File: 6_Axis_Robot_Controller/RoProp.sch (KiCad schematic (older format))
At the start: 31 parts

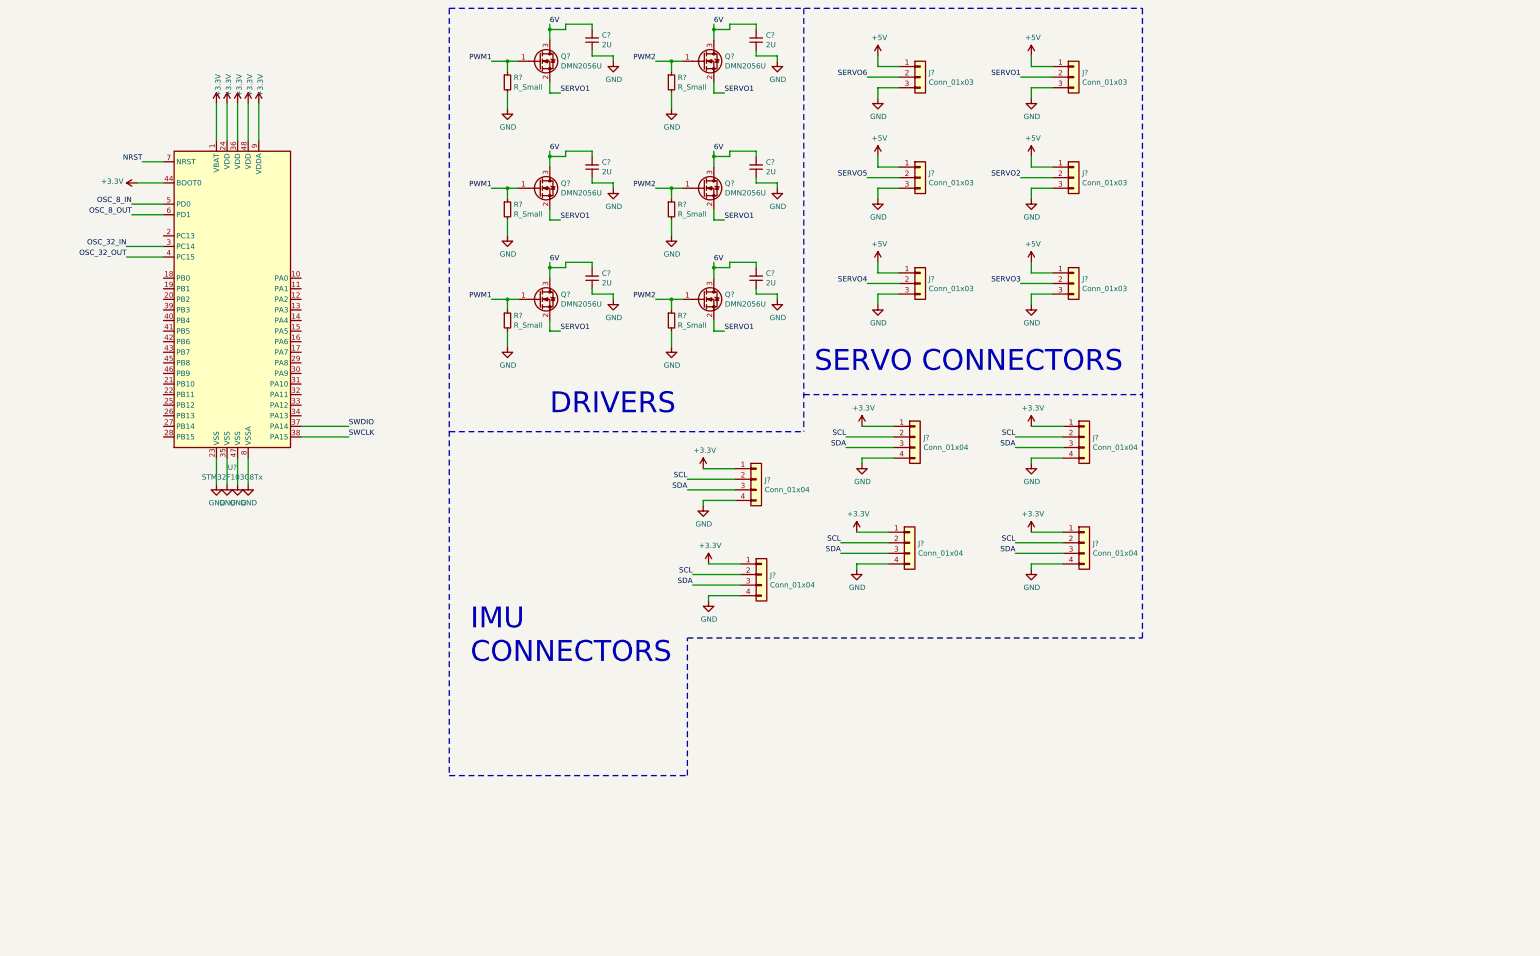
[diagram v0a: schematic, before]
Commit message: Add files via upload
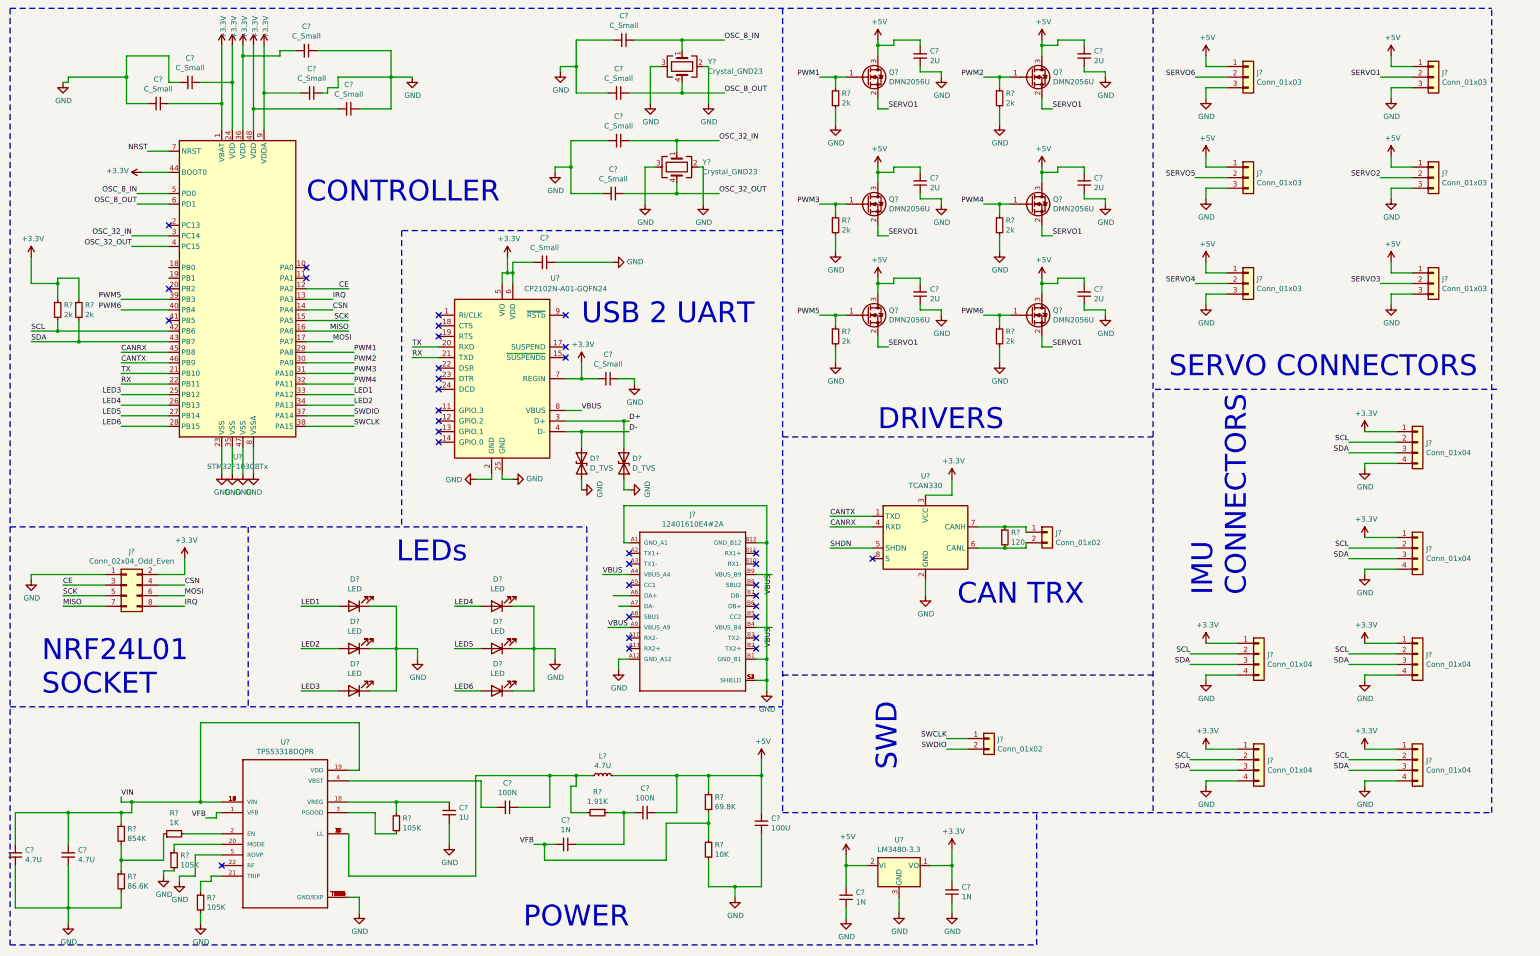
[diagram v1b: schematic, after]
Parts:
- added C? (x5): C_Small, Capacitor_SMD:C_0402_1005Metric, symbol Device:C_Small
- added C? (x2): 100N, symbol Device:C_Small
- added C? (x3): 1N, symbol Device:C_Small
- added C?: 100U, symbol Device:C_Small
- added C? (x2): 4.7U, symbol Device:C_Small
- added C?: 1U, symbol Device:C_Small
- added C? (x6): C_Small, symbol Device:C_Small
- added D? (x2): D_TVS, symbol Device:D_TVS
- added D? (x6): LED, symbol Device:LED
- added J? (x2): Conn_01x02, Connector_JST:JST_PH_B2B-PH-K_1x02_P2.00mm_Vertical, symbol Connector_Generic:Conn_01x02
- added J?: 12401610E4#2A, AMPHENOL_12401610E4#2A, symbol K_USB_C_receptacle:12401610E4#2A
- added J?: Conn_02x04_Odd_Even, symbol Connector_Generic:Conn_02x04_Odd_Even
- added L?: 4.7U, symbol Device:L_Small
- added R? (x2): 2k, Resistor_SMD:R_0805_2012Metric_Pad1.15x1.40mm_HandSolder, symbol Device:R_Small
- added R?: 1.91K, symbol Device:R_Small
- added R?: 69.8K, symbol Device:R_Small
- added R?: 10K, symbol Device:R_Small
- added R?: 1K, symbol Device:R_Small
- added R?: 854K, symbol Device:R_Small
- added R?: 86.6K, symbol Device:R_Small
- added R? (x3): 105K, symbol Device:R_Small
- added R?: 120, symbol Device:R_Small
- added U?: TPS53318DQPR, CONV_TPS53318DQPR, symbol K_TPS53318DQPR:TPS53318DQPR
- added U?: LM3480-3.3, Package_TO_SOT_SMD:SOT-23, symbol Regulator_Linear:LM3480-3.3
- added U?: TCAN330, symbol Interface_CAN_LIN:TCAN330
- added U?: CP2102N-A01-GQFN24, Package_DFN_QFN:QFN-24-1EP_4x4mm_P0.5mm_EP2.6x2.6mm, symbol Interface_USB:CP2102N-A01-GQFN24
- added Y? (x2): Crystal_GND23, symbol Device:Crystal_GND23
- R? (x6): value R_Small -> 2k
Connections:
- net 6V is gone; now on net +5V: C?.2, C?.2, C?.2, C?.2, C?.2, C?.2, Q?.3 (D), Q?.3 (D), Q?.3 (D), Q?.3 (D), Q?.3 (D), Q?.3 (D)
- net +3V3: now also C?.1, C?.1, C?.2, C?.2, C?.2, C?.2, C?.2, C?.2, J?.2 (Pin_2), R?.1, R?.1, U?.1 (VO), U?.3 (VCC), U?.5 (VIO), U?.6 (VDD), U?.7 (REGIN)
- net +5V: now also C?.1, C?.2, C?.2, L?.2, R?.2, U?.2 (VI)
- net GND: now also C?.1, C?.1, C?.1, C?.1, C?.1, C?.1, C?.1, C?.1, C?.1, C?.1, C?.1, C?.2, C?.2, C?.2, C?.2, C?.2, C?.2, D?.1 (K), D?.1 (K), D?.1 (K), D?.1 (K), D?.1 (K), D?.1 (K), D?.2 (A2), D?.2 (A2), J?.1 (Pin_1), J?.A1 (GND_A1), J?.A12 (GND_A12), J?.B1 (GND_B1), J?.B12 (GND_B12), J?.S1 (SHIELD), J?.S2 (SHIELD), J?.S3 (SHIELD), J?.S4 (SHIELD), R?.1, R?.2, R?.2, R?.2, U?.2 (GND), U?.2 (GND), U?.23 (GND/EXP), U?.25 (GND), U?.3 (GND), U?.5 (ROVP), U?.TV1 (GND/EXP), U?.TV10 (GND/EXP), U?.TV11 (GND/EXP), U?.TV12 (GND/EXP), U?.TV13 (GND/EXP), U?.TV14 (GND/EXP), U?.TV15 (GND/EXP), U?.TV16 (GND/EXP), U?.TV17 (GND/EXP), U?.TV18 (GND/EXP), U?.TV19 (GND/EXP), U?.TV2 (GND/EXP), U?.TV20 (GND/EXP), U?.TV21 (GND/EXP), U?.TV3 (GND/EXP), U?.TV4 (GND/EXP), U?.TV5 (GND/EXP), U?.TV6 (GND/EXP), U?.TV7 (GND/EXP), U?.TV8 (GND/EXP), U?.TV9 (GND/EXP), Y?.2, Y?.2, Y?.3, Y?.3
- net OSC_32_IN: now also C?.1, Y?.1
- net OSC_32_OUT: now also C?.1, Y?.4
- net OSC_8_IN: now also C?.1, Y?.1
- net OSC_8_OUT: now also C?.1, Y?.4
- net PWM1: now also U?.29 (PA8); no longer Q?.1 (G), Q?.1 (G), R?.1, R?.1
- net PWM2: now also U?.30 (PA9); no longer Q?.1 (G), Q?.1 (G), R?.1, R?.1
- net SCL: now also U?.42 (PB6), R?.2
- net SDA: now also U?.43 (PB7), R?.2
- net SWCLK: now also J?.1 (Pin_1)
- net SWDIO: now also J?.2 (Pin_2)
- net CE: now reaches U?.12 (PA2)
- net CE: now also J?.3 (Pin_3)
- net IRQ: now reaches U?.13 (PA3)
- net IRQ: now also J?.8 (Pin_8)
- net CSN: now reaches U?.14 (PA4)
- net CSN: now also J?.4 (Pin_4)
- net SCK: now reaches U?.15 (PA5)
- net SCK: now also J?.5 (Pin_5)
- net MISO: now reaches U?.16 (PA6)
- net MISO: now also J?.7 (Pin_7)
- net MOSI: now reaches U?.17 (PA7)
- net MOSI: now also J?.6 (Pin_6)
- net TX: now reaches U?.21 (PB10)
- net TX: now also U?.20 (RXD)
- net RX: now reaches U?.22 (PB11)
- net RX: now also U?.21 (TXD)
- net LED3: now reaches U?.25 (PB12)
- net LED3: now also D?.2 (A)
- net LED4: now reaches U?.26 (PB13)
- net LED4: now also D?.2 (A)
- net LED5: now reaches U?.27 (PB14)
- net LED5: now also D?.2 (A)
- net LED6: now reaches U?.28 (PB15)
- net LED6: now also D?.2 (A)
- net PWM3: now reaches U?.31 (PA10)
- net PWM3: now also Q?.1 (G), R?.1
- net PWM4: now reaches U?.32 (PA11)
- net PWM4: now also Q?.1 (G), R?.1
- net LED1: now reaches U?.33 (PA12)
- net LED1: now also D?.2 (A)
- net LED2: now reaches U?.34 (PA13)
- net LED2: now also D?.2 (A)
- net PWM5: now reaches U?.39 (PB3)
- net PWM5: now also Q?.1 (G), R?.1
- net PWM6: now reaches U?.40 (PB4)
- net PWM6: now also Q?.1 (G), R?.1
- net CANRX: now reaches U?.45 (PB8)
- net CANRX: now also U?.4 (RXD)
- net CANTX: now reaches U?.46 (PB9)
- net CANTX: now also U?.1 (TXD)
- new net: C?.1, L?.1, R?.2, U?.10 (LL), U?.11 (LL), U?.6 (LL), U?.7 (LL), U?.8 (LL), U?.9 (LL)
- new net: C?.2, R?.2, U?.18 (VREG)
- new net: R?.2, U?.2 (EN)
- new net: R?.1, U?.20 (MODE)
- new net: R?.1, U?.21 (TRIP)
- new net: R?.1, U?.3 (PGOOD)
- new net: C?.2, U?.4 (VBST)
- new net: C?.1, C?.2, R?.1
- new net: R?.1, R?.1, R?.2
- new net: J?.2 (Pin_2), R?.2, U?.6 (CANL)
- new net: J?.1 (Pin_1), R?.1, U?.7 (CANH)
- new net D+: D?.1 (A1), U?.3 (D+)
- new net D-: D?.1 (A1), U?.4 (D-)
- new net SHDN: U?.5 (SHDN)
- new net VBUS: J?.A4 (VBUS_A4), J?.A9 (VBUS_A9), J?.B4 (VBUS_B4), J?.B9 (VBUS_B9), U?.8 (VBUS)
- new net VFB: C?.2, R?.1, R?.2, U?.1 (VFB)
- new net VIN: C?.2, C?.2, R?.1, U?.12 (VIN), U?.13 (VIN), U?.14 (VIN), U?.15 (VIN), U?.16 (VIN), U?.17 (VIN), U?.19 (VDD)
- no-connect marks 0 -> 34
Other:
- note added: "CAN TRX"
- note added: "CONTROLLER\n"
- note added: "LEDs\n"
- note added: "NRF24L01 \nSOCKET"
- note added: "POWER \n"
- note added: "SWD\n"
- note added: "USB 2 UART"
- moved on the sheet: C?, J?, Q?, R?, U?
